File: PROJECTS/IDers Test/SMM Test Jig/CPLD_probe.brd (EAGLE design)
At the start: 24.1 x 40.3 mm, 2 parts

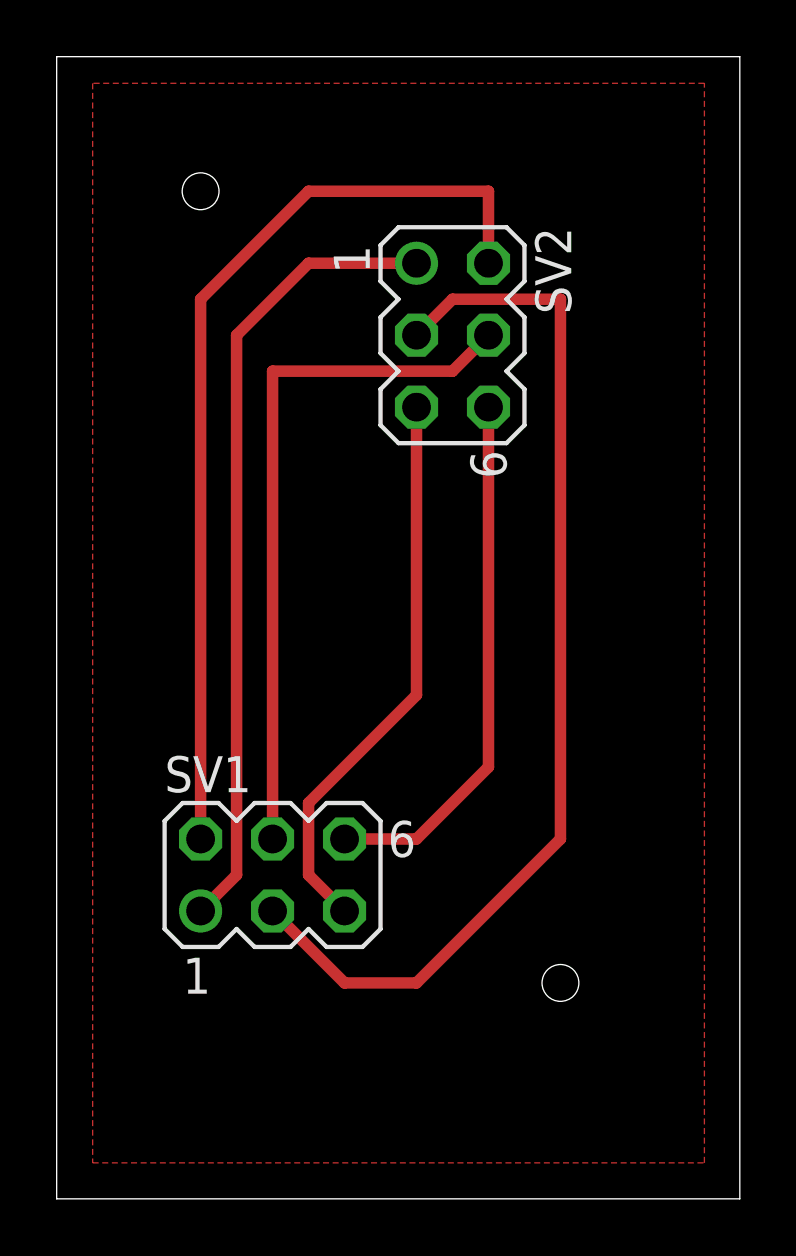
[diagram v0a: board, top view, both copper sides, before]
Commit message: update
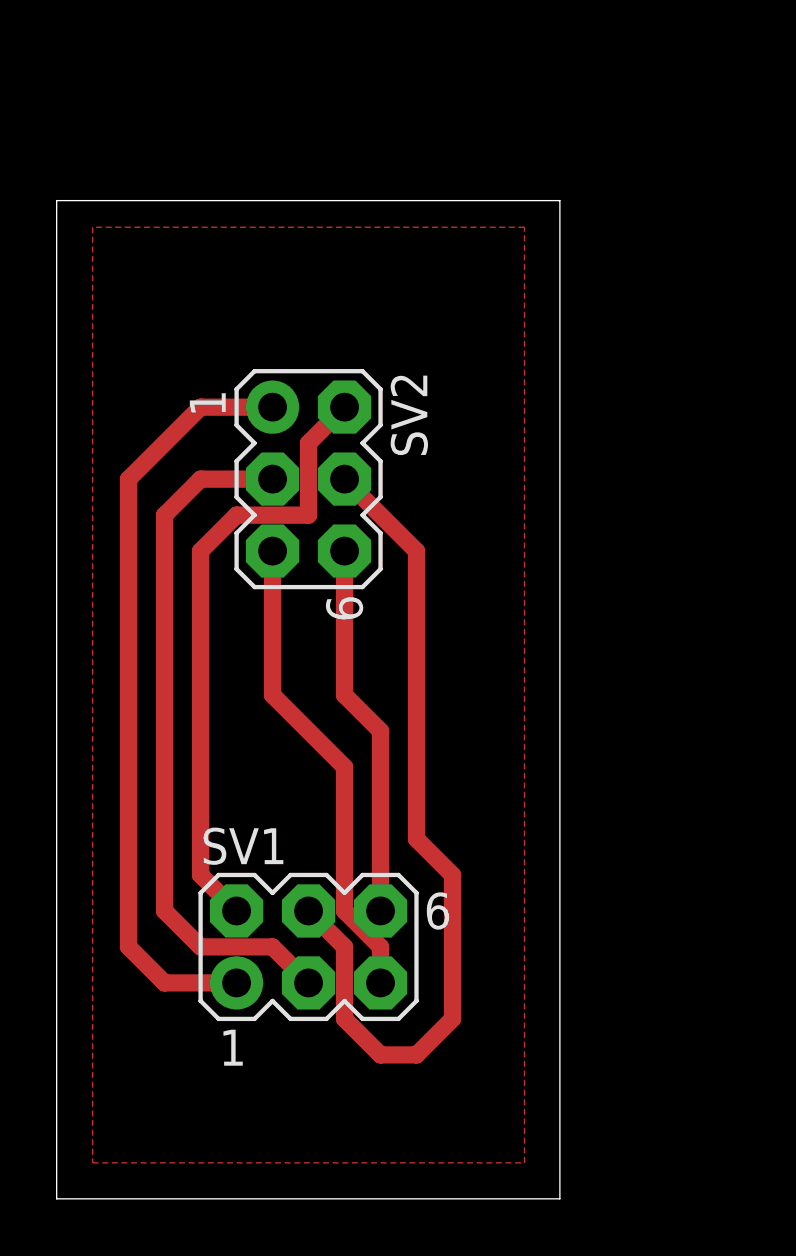
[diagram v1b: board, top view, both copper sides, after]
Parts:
- moved SV2 7.18 mm to (8.89, 25.4)
- moved SV1 2.84 mm to (8.89, 8.89)
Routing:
- net N$3: track 38.0 -> 24.4 mm
- net N$1: track 33.3 -> 21.9 mm
- net N$6: track 18.8 -> 13.2 mm
- net N$5: track 24.7 -> 29.8 mm
- net N$4: track 19.9 -> 16.8 mm
- net N$2: track 28.2 -> 27.0 mm
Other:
- board size 24.1 x 40.3 mm -> 17.8 x 35.2 mm
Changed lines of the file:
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@@
 <board>
 <plain>
-<wire x1="0" y1="0" x2="24.11" y2="0" width="0" layer="20"/>
-<wire x1="24.11" y1="0" x2="24.11" y2="40.31" width="0" layer="20"/>
-<wire x1="24.11" y1="40.31" x2="0" y2="40.31" width="0" layer="20"/>
-<wire x1="0" y1="40.31" x2="0" y2="0" width="0" layer="20"/>
-<hole x="17.78" y="7.62" drill="1.3"/>
-<hole x="5.08" y="35.56" drill="1.3"/>
-<dimension x1="24.11" y1="40.31" x2="27.94" y2="0" x3="26.67" y3="20.155" textsize="1.778" layer="25" dtype="vertical"/>
-<dimension x1="0" y1="40.31" x2="24.13" y2="43.18" x3="12.065" y3="41.91" textsize="1.778" layer="25" dtype="horizontal"/>
+<wire x1="0" y1="0" x2="17.76" y2="0" width="0" layer="20"/>
+<wire x1="17.76" y1="0" x2="17.76" y2="35.23" width="0" layer="20"/>
+<wire x1="17.76" y1="35.23" x2="0" y2="35.23" width="0" layer="20"/>
+<wire x1="0" y1="35.23" x2="0" y2="0" width="0" layer="20"/>
+<dimension x1="17.76" y1="0" x2="17.76" y2="35.23" x3="22.86" y3="17.615" textsize="1.778" layer="20"/>
+<dimension x1="0" y1="0" x2="17.76" y2="0" x3="8.88" y3="-3.81" textsize="1.778" layer="20"/>
 </plain>
 <attributes>
@@
 <param name="rvMicroViaOuter" value="0.25"/>
 <param name="rvMicroViaInner" value="0.25"/>
-<param name="rlMinPadTop" value="10mil"/>
+<param name="rlMinPadTop" value="17mil"/>
 <param name="rlMaxPadTop" value="20mil"/>
 <param name="rlMinPadInner" value="10mil"/>
@@
 </autorouter>
 <elements>
-<element name="SV1" library="con-lstb" package="MA03-2" value="" x="7.62" y="11.43">
-<attribute name="OC_NEWARK" value="unknown" x="7.62" y="11.43" size="1.778" layer="27" display="off"/>
-<attribute name="MPN" value="" x="7.62" y="11.43" size="1.778" layer="27" display="off"/>
-<attribute name="MF" value="" x="7.62" y="11.43" size="1.778" layer="27" display="off"/>
-<attribute name="OC_FARNELL" value="unknown" x="7.62" y="11.43" size="1.778" layer="27" display="off"/>
+<element name="SV1" library="con-lstb" package="MA03-2" value="" x="8.89" y="8.89">
+<attribute name="OC_NEWARK" value="unknown" x="8.89" y="8.89" size="1.778" layer="27" display="off"/>
+<attribute name="MPN" value="" x="8.89" y="8.89" size="1.778" layer="27" display="off"/>
+<attribute name="MF" value="" x="8.89" y="8.89" size="1.778" layer="27" display="off"/>
+<attribute name="OC_FARNELL" value="unknown" x="8.89" y="8.89" size="1.778" layer="27" display="off"/>
 </element>
-<element name="SV2" library="con-lstb" package="MA03-2" value="" x="13.97" y="30.48" rot="R270">
-<attribute name="OC_NEWARK" value="unknown" x="13.97" y="30.48" size="1.778" layer="27" rot="R270" display="off"/>
-<attribute name="MPN" value="" x="13.97" y="30.48" size="1.778" layer="27" rot="R270" display="off"/>
-<attribute name="MF" value="" x="13.97" y="30.48" size="1.778" layer="27" rot="R270" display="off"/>
-<attribute name="OC_FARNELL" value="unknown" x="13.97" y="30.48" size="1.778" layer="27" rot="R270" display="off"/>
+<element name="SV2" library="con-lstb" package="MA03-2" value="" x="8.89" y="25.4" rot="R270">
+<attribute name="OC_NEWARK" value="unknown" x="8.89" y="25.4" size="1.778" layer="27" rot="R270" display="off"/>
+<attribute name="MPN" value="" x="8.89" y="25.4" size="1.778" layer="27" rot="R270" display="off"/>
+<attribute name="MF" value="" x="8.89" y="25.4" size="1.778" layer="27" rot="R270" display="off"/>
+<attribute name="OC_FARNELL" value="unknown" x="8.89" y="25.4" size="1.778" layer="27" rot="R270" display="off"/>
 </element>
 </elements>
@@
 <contactref element="SV2" pad="2"/>
 <contactref element="SV1" pad="2"/>
-<wire x1="5.08" y1="12.7" x2="5.08" y2="31.75" width="0.4064" layer="1"/>
-<wire x1="5.08" y1="31.75" x2="8.89" y2="35.56" width="0.4064" layer="1"/>
-<wire x1="8.89" y1="35.56" x2="15.24" y2="35.56" width="0.4064" layer="1"/>
-<wire x1="15.24" y1="35.56" x2="15.24" y2="33.02" width="0.4064" layer="1"/>
+<wire x1="10.16" y1="27.94" x2="8.89" y2="26.67" width="0.6096" layer="1"/>
+<wire x1="6.35" y1="24.13" x2="5.08" y2="22.86" width="0.6096" layer="1"/>
+<wire x1="5.08" y1="22.86" x2="5.08" y2="11.43" width="0.6096" layer="1"/>
+<wire x1="5.08" y1="11.43" x2="6.35" y2="10.16" width="0.6096" layer="1"/>
+<wire x1="8.89" y1="26.67" x2="8.89" y2="24.13" width="0.6096" layer="1"/>
+<wire x1="8.89" y1="24.13" x2="6.35" y2="24.13" width="0.6096" layer="1"/>
 </signal>
 <signal name="N$2">
 <contactref element="SV2" pad="1"/>
 <contactref element="SV1" pad="1"/>
-<wire x1="5.08" y1="10.16" x2="6.35" y2="11.43" width="0.4064" layer="1"/>
-<wire x1="6.35" y1="11.43" x2="6.35" y2="30.48" width="0.4064" layer="1"/>
-<wire x1="6.35" y1="30.48" x2="8.89" y2="33.02" width="0.4064" layer="1"/>
-<wire x1="8.89" y1="33.02" x2="12.7" y2="33.02" width="0.4064" layer="1"/>
+<wire x1="7.62" y1="27.94" x2="5.08" y2="27.94" width="0.6096" layer="1"/>
+<wire x1="5.08" y1="27.94" x2="2.54" y2="25.4" width="0.6096" layer="1"/>
+<wire x1="2.54" y1="25.4" x2="2.54" y2="8.89" width="0.6096" layer="1"/>
+<wire x1="2.54" y1="8.89" x2="3.81" y2="7.62" width="0.6096" layer="1"/>
+<wire x1="3.81" y1="7.62" x2="6.35" y2="7.62" width="0.6096" layer="1"/>
 </signal>
 <signal name="N$3">
 <contactref element="SV2" pad="3"/>
 <contactref element="SV1" pad="3"/>
-<wire x1="7.62" y1="10.16" x2="10.16" y2="7.62" width="0.4064" layer="1"/>
-<wire x1="10.16" y1="7.62" x2="12.7" y2="7.62" width="0.4064" layer="1"/>
-<wire x1="12.7" y1="7.62" x2="17.78" y2="12.7" width="0.4064" layer="1"/>
-<wire x1="17.78" y1="12.7" x2="17.78" y2="31.75" width="0.4064" layer="1"/>
-<wire x1="17.78" y1="31.75" x2="13.97" y2="31.75" width="0.4064" layer="1"/>
-<wire x1="13.97" y1="31.75" x2="12.7" y2="30.48" width="0.4064" layer="1"/>
+<wire x1="7.62" y1="25.4" x2="5.08" y2="25.4" width="0.6096" layer="1"/>
+<wire x1="5.08" y1="25.4" x2="3.81" y2="24.13" width="0.6096" layer="1"/>
+<wire x1="3.81" y1="24.13" x2="3.81" y2="10.16" width="0.6096" layer="1"/>
+<wire x1="3.81" y1="10.16" x2="5.08" y2="8.89" width="0.6096" layer="1"/>
+<wire x1="5.08" y1="8.89" x2="7.62" y2="8.89" width="0.6096" layer="1"/>
+<wire x1="7.62" y1="8.89" x2="8.89" y2="7.62" width="0.6096" layer="1"/>
 </signal>
 <signal name="N$4">
 <contactref element="SV2" pad="5"/>
 <contactref element="SV1" pad="5"/>
-<wire x1="10.16" y1="10.16" x2="8.89" y2="11.43" width="0.4064" layer="1"/>
-<wire x1="8.89" y1="11.43" x2="8.89" y2="13.97" width="0.4064" layer="1"/>
-<wire x1="8.89" y1="13.97" x2="12.7" y2="17.78" width="0.4064" layer="1"/>
-<wire x1="12.7" y1="17.78" x2="12.7" y2="27.94" width="0.4064" layer="1"/>
+<wire x1="7.62" y1="22.86" x2="7.62" y2="17.78" width="0.6096" layer="1"/>
+<wire x1="7.62" y1="17.78" x2="10.16" y2="15.24" width="0.6096" layer="1"/>
+<wire x1="10.16" y1="15.24" x2="10.16" y2="10.16" width="0.6096" layer="1"/>
+<wire x1="10.16" y1="10.16" x2="11.43" y2="8.89" width="0.6096" layer="1"/>
+<wire x1="11.43" y1="8.89" x2="11.43" y2="7.62" width="0.6096" layer="1"/>
 </signal>
 <signal name="N$5">
 <contactref element="SV2" pad="4"/>
 <contactref element="SV1" pad="4"/>
-<wire x1="7.62" y1="12.7" x2="7.62" y2="29.21" width="0.4064" layer="1"/>
-<wire x1="7.62" y1="29.21" x2="13.97" y2="29.21" width="0.4064" layer="1"/>
-<wire x1="13.97" y1="29.21" x2="15.24" y2="30.48" width="0.4064" layer="1"/>
+<wire x1="10.16" y1="25.4" x2="12.7" y2="22.86" width="0.6096" layer="1"/>
+<wire x1="12.7" y1="22.86" x2="12.7" y2="12.7" width="0.6096" layer="1"/>
+<wire x1="12.7" y1="12.7" x2="13.97" y2="11.43" width="0.6096" layer="1"/>
+<wire x1="13.97" y1="11.43" x2="13.97" y2="6.35" width="0.6096" layer="1"/>
+<wire x1="13.97" y1="6.35" x2="12.7" y2="5.08" width="0.6096" layer="1"/>
+<wire x1="12.7" y1="5.08" x2="11.43" y2="5.08" width="0.6096" layer="1"/>
+<wire x1="11.43" y1="5.08" x2="10.16" y2="6.35" width="0.6096" layer="1"/>
+<wire x1="10.16" y1="6.35" x2="10.16" y2="8.89" width="0.6096" layer="1"/>
+<wire x1="10.16" y1="8.89" x2="8.89" y2="10.16" width="0.6096" layer="1"/>
 </signal>
 <signal name="N$6">
 <contactref element="SV2" pad="6"/>
 <contactref element="SV1" pad="6"/>
-<wire x1="15.24" y1="27.94" x2="15.24" y2="15.24" width="0.4064" layer="1"/>
-<wire x1="15.24" y1="15.24" x2="12.7" y2="12.7" width="0.4064" layer="1"/>
-<wire x1="12.7" y1="12.7" x2="10.16" y2="12.7" width="0.4064" layer="1"/>
+<wire x1="10.16" y1="22.86" x2="10.16" y2="17.78" width="0.6096" layer="1"/>
+<wire x1="10.16" y1="17.78" x2="11.43" y2="16.51" width="0.6096" layer="1"/>
+<wire x1="11.43" y1="16.51" x2="11.43" y2="10.16" width="0.6096" layer="1"/>
 </signal>
 <signal name="GND">
 <polygon width="0.4064" layer="1">
-<vertex x="1.27" y="39.37"/>
+<vertex x="1.27" y="34.29"/>
 <vertex x="1.27" y="1.27"/>
-<vertex x="22.86" y="1.27"/>
-<vertex x="22.86" y="39.37"/>
+<vertex x="16.51" y="1.27"/>
+<vertex x="16.51" y="34.29"/>
 </polygon>
 </signal>
